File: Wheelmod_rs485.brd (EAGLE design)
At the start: 42 x 40 mm, 52 parts, among them IC1 SN75176BPSR, SW1 RST_SW, SW2 HWB_SW, U1 ATMEGA8U2AU, U2 SI8441IS1, U3 MC33887-HSOP, U4 NFET-SOIC8, U5 LDO, X1 MINI-USB, X3 ENC, X5 LOGIC_IN, Y1 SMDRESONATOR

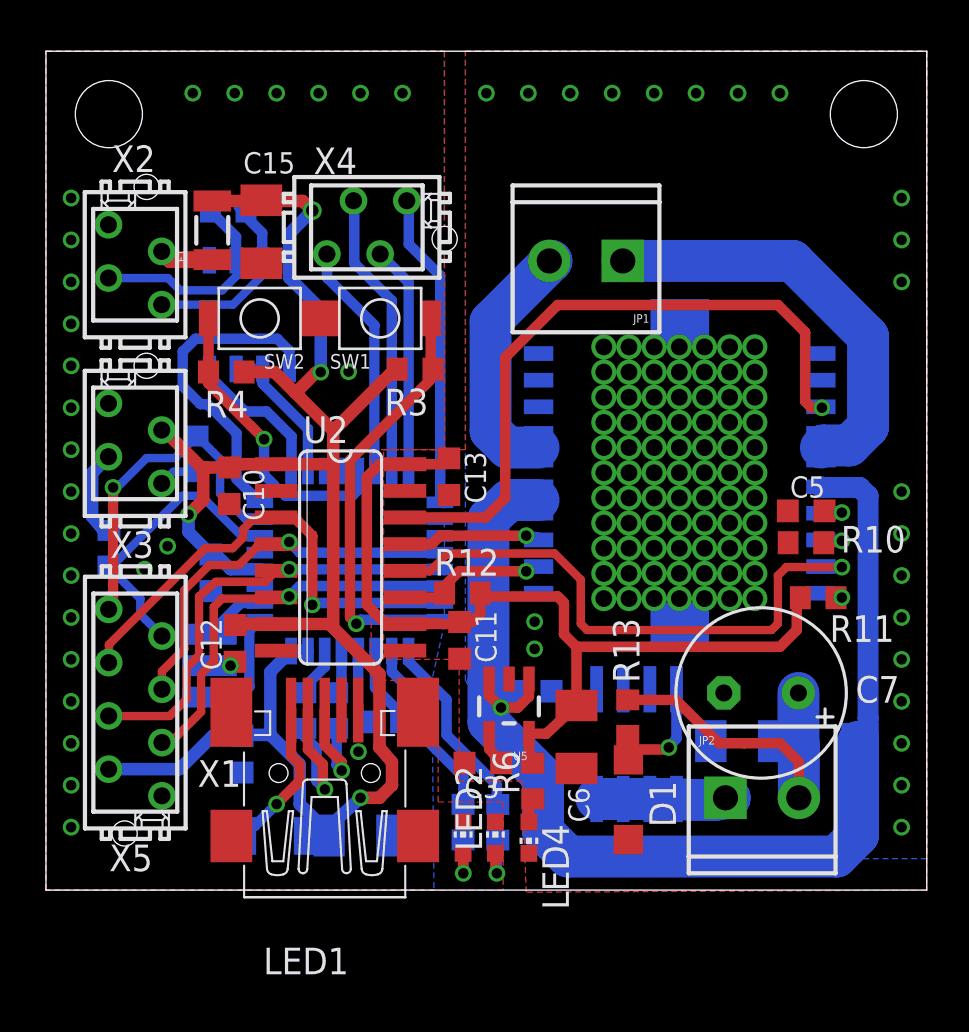
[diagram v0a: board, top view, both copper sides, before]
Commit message: Added fixes to Tiina's version
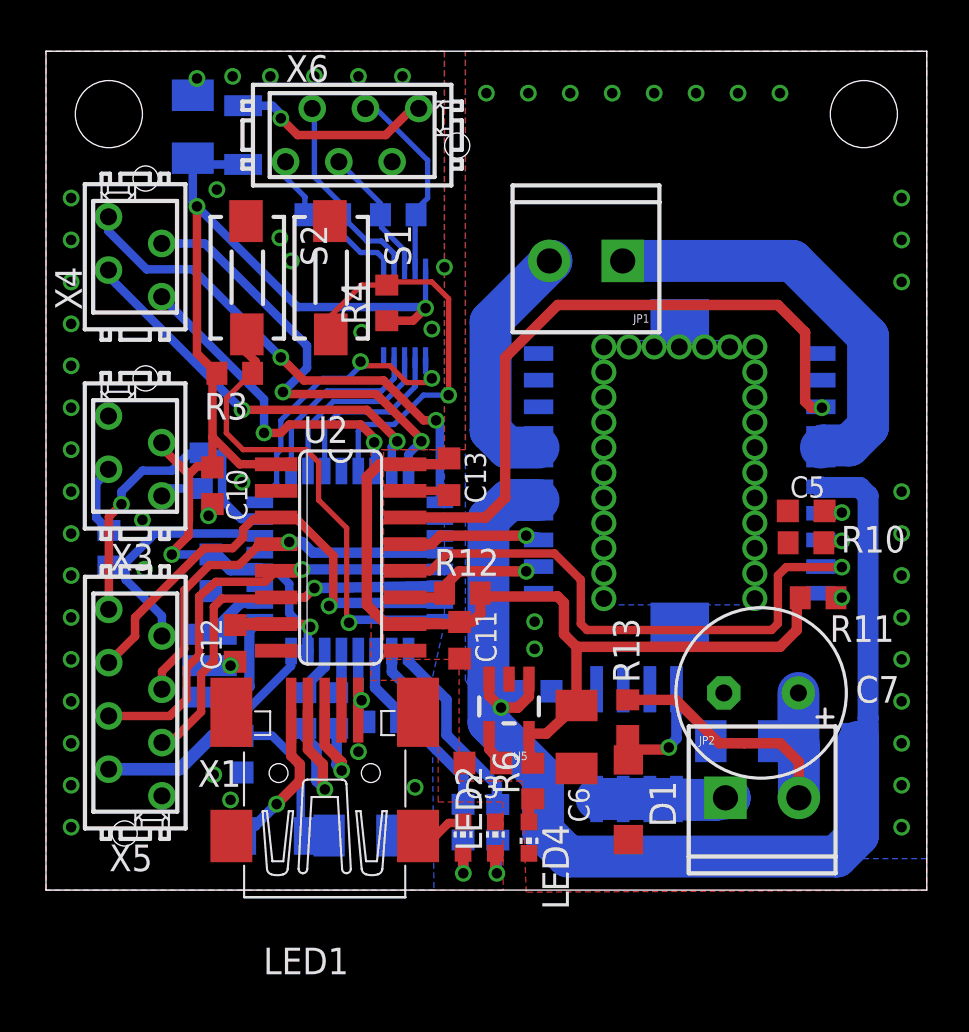
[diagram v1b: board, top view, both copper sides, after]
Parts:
- removed IC1: SN75176BPSR, rs485DRIVER:SO8
- removed SW1: RST_SW, Erik:SMD-TACT-3.9X2.9
- removed SW2: HWB_SW, Erik:SMD-TACT-3.9X2.9
- removed X2: (no value), con-amp-micromatch:MICROMATCH-4
- added R9: 120, rcl:R0603
- added S1: HWB, kommunikatsioonimoodul:ADTSM3
- added S2: RESET, kommunikatsioonimoodul:ADTSM3
- added U$1: SN65HVF76DGS, rs485:MSOP10
- added X6: R485-IO, con-amp-micromatch:MICROMATCH-6
- moved X4 11.1 mm to (4.25, 30.2), turned to 90 degrees
- moved R3 8.60 mm to (9.00, 24.6)
- moved R4 8.33 mm to (16.2, 28.0), turned to 270 degrees
- moved R5 8.11 mm to (16.8, 32.2)
- moved C15 5.98 mm to (7.00, 36.4), flipped to the bottom, turned to 90 degrees
- moved F1 4.77 mm to (9.40, 36.0), flipped to the bottom, turned to 270 degrees
- moved R17 0.82 mm to (7.40, 20.0)
- moved C10 0.80 mm to (7.94, 19.3)
- moved X3 0.60 mm to (4.25, 20.7)
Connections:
- removed net N$32: F1.1, X2.2
- new net N$33: F1.1, X6.1
- new net RE: U$1.2, U1.11
- new net Y: R9.1, U$1.6, X6.6
- new net Z: R9.2, U$1.7, X6.5
- net A: now also R5.2, U$1.9, X6.3; no longer IC1.6, R5.1, X2.3
- net B: now also R5.1, U$1.8, X6.4; no longer IC1.7, R5.2, X2.4
- net DE: now also U$1.3; no longer IC1.2, IC1.3
- net GND: now also S1.1, S2.1, U$1.5, X6.2; no longer IC1.5, SW1.1, SW2.2, X2.1
- net N$10: now also S2.2; no longer SW1.2
- net N$2: now also S1.2; no longer SW2.1
- net RX: now also U$1.1; no longer IC1.1
- net TX: now also U$1.4; no longer IC1.4
- net VCC: now also U$1.10; no longer IC1.8
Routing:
- net N$27: track 10.9 -> 20.9 mm, vias 0 -> 2
- net Z: track 0.00 -> 9.68 mm
- net N$33: track 0.00 -> 9.60 mm, vias 0 -> 1
- net N$31: track 15.0 -> 24.0 mm, vias 0 -> 2
- net VCC: track 92.9 -> 84.0 mm
- net RE: track 0.00 -> 8.60 mm
- net Y: track 0.00 -> 8.04 mm
- net N$26: track 13.6 -> 18.9 mm, vias 0 -> 2
- net N$2: track 14.5 -> 19.0 mm
- net N$24: track 11.3 -> 15.8 mm, vias 0 -> 2
- net B: track 9.21 -> 6.42 mm
- net N$10: track 20.4 -> 23.1 mm
- net N$32: track 2.57 -> 0.00 mm
- net GND: track 5.51 -> 7.94 mm, vias 27 -> 38
- net GNDA: track 0.03 -> 2.21 mm, vias 99 -> 49
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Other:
- board text added: "v0.8"
- board text removed: "v0.7"
